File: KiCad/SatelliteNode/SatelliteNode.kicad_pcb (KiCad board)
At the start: 2 copper layers, 3.2 x 25.2 mm, 5 parts, among them J1 Isolated_RS485, J2 Conn_01x04, U2 NJM2845DL1-05, U4 MCP23017_SP

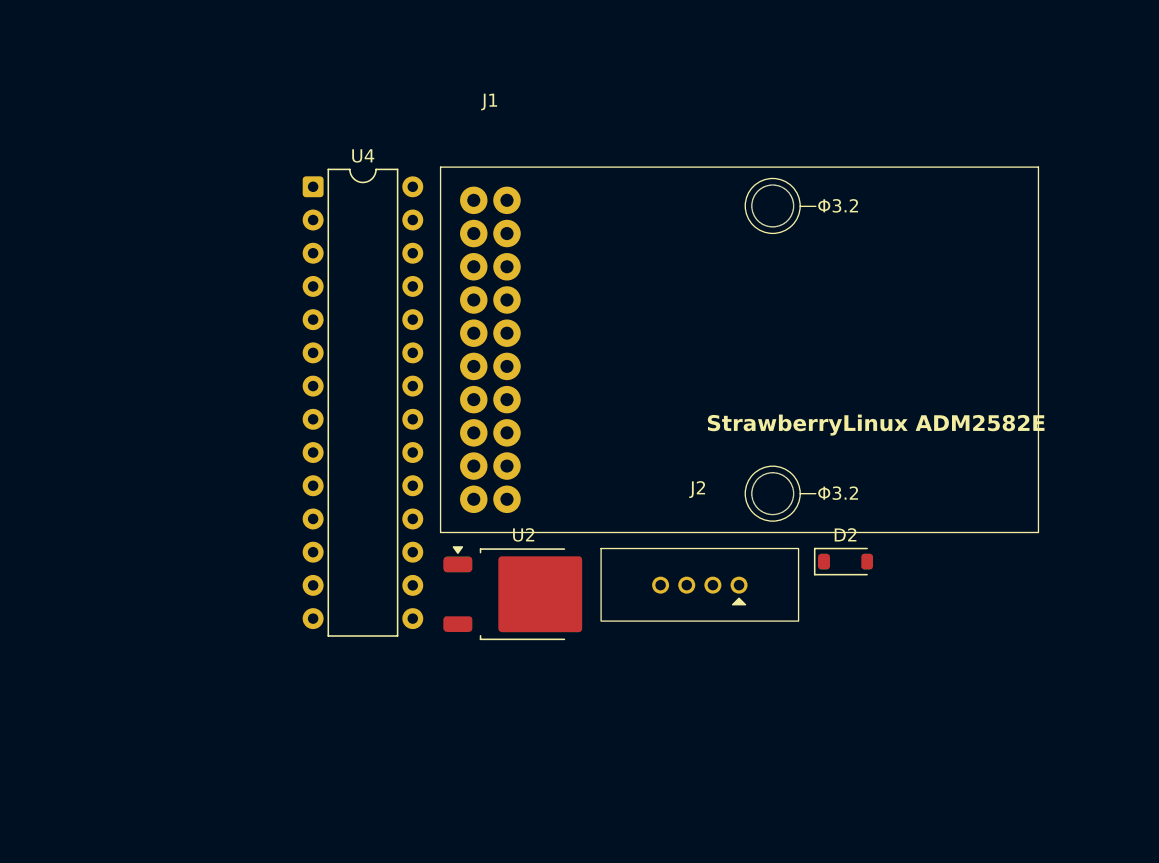
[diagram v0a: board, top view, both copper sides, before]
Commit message: SatelliteNode Build-1を発行
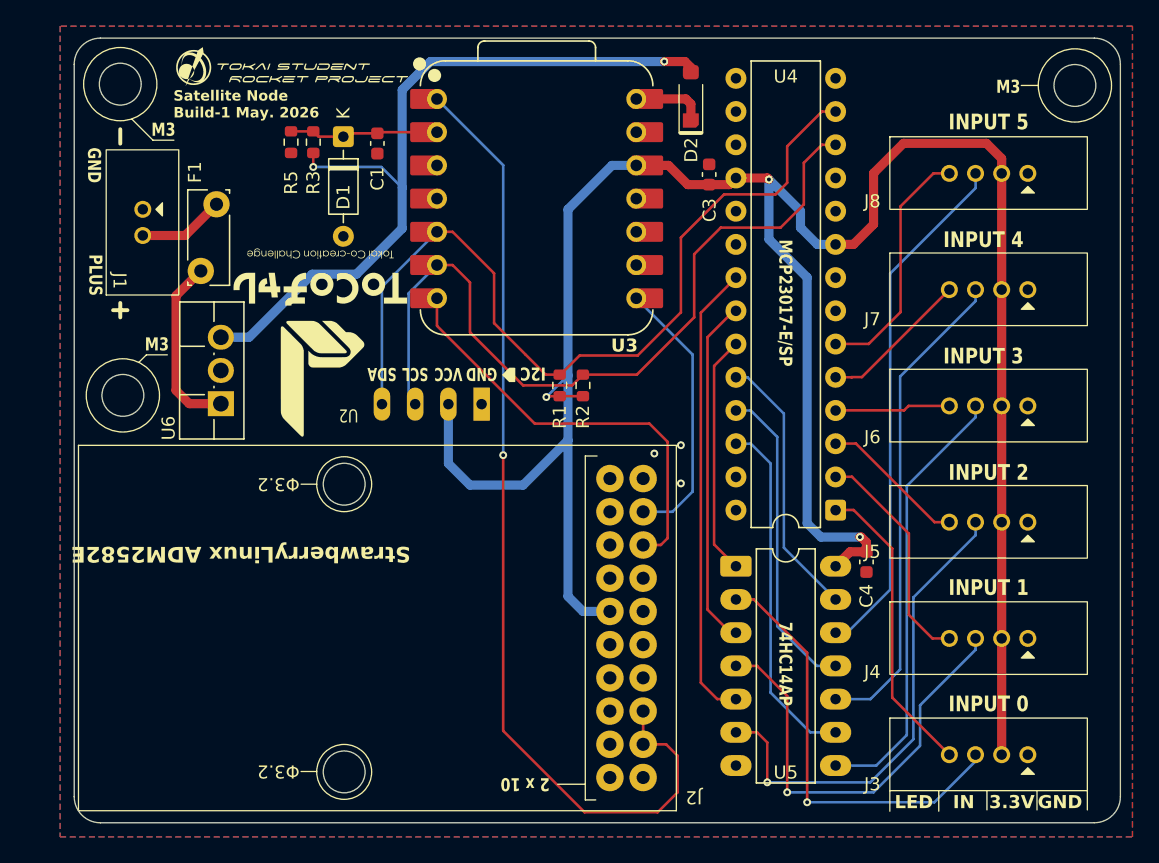
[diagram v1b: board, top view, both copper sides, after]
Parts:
- added C1: 0.1uF, Capacitor_SMD:C_0603_1608Metric, F.Cu at (90.2, 73.1)
- added C3: 0.1uF, Capacitor_SMD:C_0603_1608Metric, F.Cu at (115.6, 75.4)
- added C4: 0.1uF, Capacitor_SMD:C_0603_1608Metric, F.Cu at (127.6, 105.1)
- added D1: BZX55C3V3, Diode_THT:D_DO-35_SOD27_P7.62mm_Horizontal, F.Cu at (87.6, 72.5)
- added F1: MF-R050, Fuse:Fuse_Bourns_MF-RG300, F.Cu at (77.9, 77.7)
- added G***: LOGO, LOGO, F.Cu at (83.7, 67.2)
- added G***: LOGO, LOGO, F.Cu at (85.8, 88.4)
- added H1: MountingHole, MountingHole:MountingHole_3.2mm_M3, F.Cu at (70.7, 92.3)
- added H2: MountingHole, MountingHole:MountingHole_3.2mm_M3, F.Cu at (143.5, 68.6)
- added H3: MountingHole, MountingHole:MountingHole_3.2mm_M3, F.Cu at (70.5, 68.5)
- added J3: Conn_01x04, TSRP_Connector_Hirose:DF51A-4P-2DSA, F.Cu at (136.9, 122.4)
- added J4: Conn_01x04, TSRP_Connector_Hirose:DF51A-4P-2DSA, F.Cu at (136.9, 113.5)
- added J5: Conn_01x04, TSRP_Connector_Hirose:DF51A-4P-2DSA, F.Cu at (136.9, 104.6)
- added J6: Conn_01x04, TSRP_Connector_Hirose:DF51A-4P-2DSA, F.Cu at (136.9, 95.7)
- added J7: Conn_01x04, TSRP_Connector_Hirose:DF51A-4P-2DSA, F.Cu at (136.9, 86.8)
- added J8: Conn_01x04, TSRP_Connector_Hirose:DF51A-4P-2DSA, F.Cu at (136.9, 77.9)
- added R1: 4.7kR, Resistor_SMD:R_0603_1608Metric, F.Cu at (104.1, 91.6)
- added R2: 4.7kR, Resistor_SMD:R_0603_1608Metric, F.Cu at (105.9, 91.6)
- added R3: 10kR 1%, Resistor_SMD:R_0603_1608Metric, F.Cu at (85.3, 73.0)
- added R5: 10kR 1%, Resistor_SMD:R_0603_1608Metric, F.Cu at (83.6, 73.0)
- added U3: XIAO-ESP32-C6, TSRP_Seeed_XIAO:XIAO-ESP32-C6-DIP, F.Cu at (102.4, 77.3)
- added U5: 74HC14, Package_DIP:DIP-14_W7.62mm_LongPads, F.Cu at (117.6, 105.4)
- added U6: BP5293-50, Package_TO_SOT_THT:TO-220F-3_Vertical, F.Cu at (78.2, 93.0)
- D2: value 1N4148W -> RB160M-30TR; footprint Diode_SMD:D_SOD-123 -> TSRP_Diode:SOD-123FL_Handsolder
- J1: value Isolated_RS485 -> 12V_Connector; footprint TSRP_IC:StrawberryLinux_ADM2582 -> TSRP_Connector_Hirose:DF51A-2P-2DSA
- J2: value Conn_01x04 -> Isolated_RS485; footprint TSRP_Connector_Hirose:DF51A-4P-2DSA -> TSRP_IC:StrawberryLinux_ADM2582
- U2: value NJM2845DL1-05 -> SSD1306; footprint Package_TO_SOT_SMD:TO-252-2 -> TSRP_IC:SSD1306
- moved U4 47.0 mm to (125.2, 101.1), turned to 180 degrees
- moved D2 37.5 mm to (114.2, 69.5), turned to 90 degrees
- moved J1 25.9 mm to (74.8, 79.1), turned to 90 degrees
- moved U2 14.9 mm to (98.2, 93.0), turned to 180 degrees
- moved J2 5.65 mm to (109.2, 110.1), turned to 180 degrees
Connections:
- D2 pad 1: +12V -> Net-(D2-K)
- J1 pad 1: unconnected-(J1-Pin_1-Pad1) -> GND
- J1 pad 2: unconnected-(J1-Pin_2-Pad2) -> +12V
- J2 pad 1: GND -> unconnected-(J2-Pin_1-Pad1)
- J2 pad 2: +3.3V -> unconnected-(J2-Pin_2-Pad2)
- J2 pad 3: Net-(J2-Pin_3) -> RS485_RO
- J2 pad 4: LED_CTL_0 -> unconnected-(J2-Pin_4-Pad4)
- U2 pad 1: +12V -> GND
- U2 pad 2: GND -> +3.3V
- U2 pad 3: +5V -> I2C_SCL
- U4 pad 21: Switch_Out_0 -> Switch_Out_2
- U4 pad 23: Switch_Out_2 -> Switch_Out_0
- U4 pad 24: Switch_Out_3 -> Switch_Out_5
- U4 pad 26: Switch_Out_5 -> Switch_Out_3
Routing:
- net +3.3V: track 0.00 -> 180.2 mm, vias 0 -> 3
- net RS485_~{RE}_DE: track 0.00 -> 75.3 mm, vias 0 -> 1
- net I2C_SDA: track 0.00 -> 65.5 mm
- net I2C_SCL: track 0.00 -> 60.6 mm
- net +5V: track 0.00 -> 60.0 mm, vias 0 -> 2
- net Net-(J8-Pin_3): track 0.00 -> 40.1 mm
- net Net-(J7-Pin_3): track 0.00 -> 37.3 mm
- net Net-(J5-Pin_3): track 0.00 -> 36.9 mm, vias 0 -> 1
- net Switch_Out_2: track 0.00 -> 35.3 mm
- net Net-(J4-Pin_3): track 0.00 -> 33.8 mm, vias 0 -> 1
- net Net-(J6-Pin_3): track 0.00 -> 33.8 mm
- net Net-(J3-Pin_3): track 0.00 -> 33.2 mm, vias 0 -> 1
- net RS485_DI: track 0.00 -> 32.9 mm
- net Switch_Out_3: track 0.00 -> 27.0 mm
- net Switch_Out_1: track 0.00 -> 26.7 mm
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- added copper zone on B.Cu, net GND
- added copper zone on F.Cu, net GND
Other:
- board size 3.2 x 25.2 mm -> 80 x 60 mm
- board text added: "2 x 10"
- board text added: "3.3V"
- board text added: "60"
- board text added: "74HC14AP"
- board text added: "80"
- board text added: "GND"
- board text added: "I2C"
- board text added: "IN"
- board text added: "INPUT 0"
- board text added: "INPUT 1"
- board text added: "INPUT 2"
- board text added: "INPUT 3"
- board text added: "INPUT 4"
- board text added: "INPUT 5"
- board text added: "LED"
- board text added: "M3"
- board text added: "MCP23017-E/SP"
- board text added: "PLUS"
- board text added: "Satellite Node Build-1 May. 2026"
- board text added: "リセッタブルヒューズ トリップ電流:1A"
